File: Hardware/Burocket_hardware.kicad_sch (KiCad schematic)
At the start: 0 parts

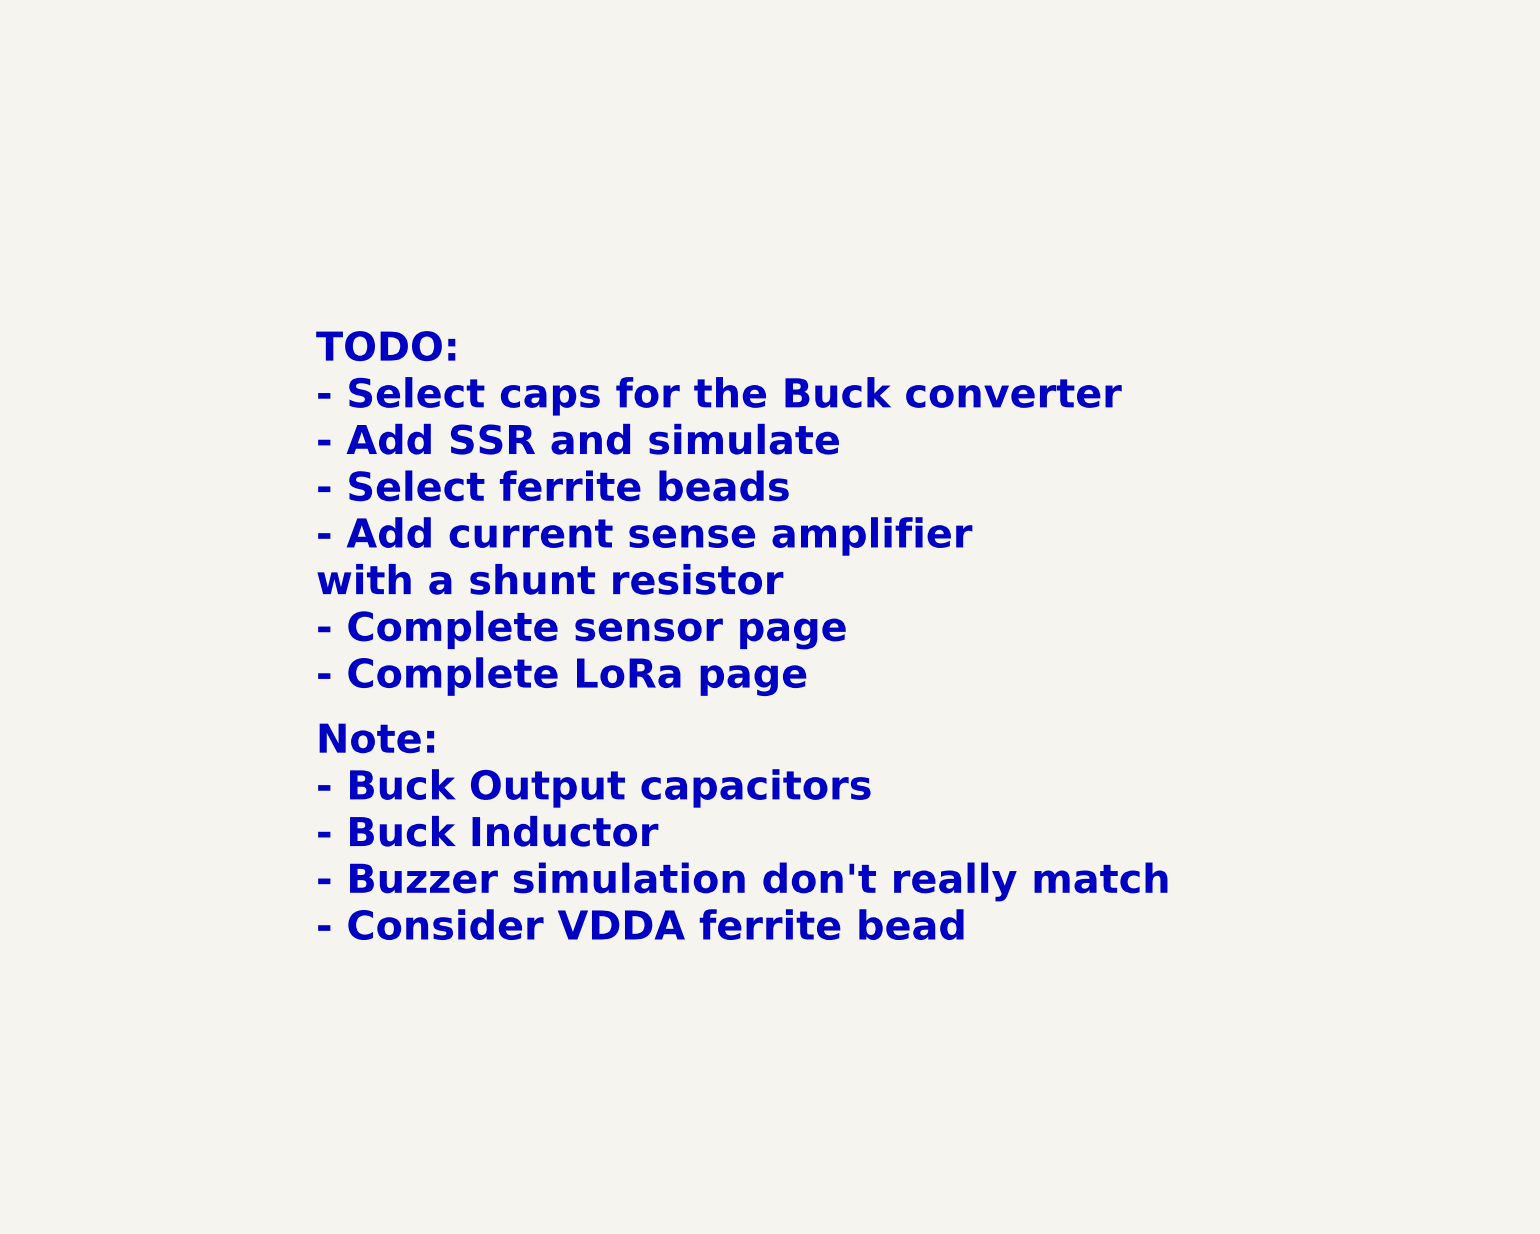
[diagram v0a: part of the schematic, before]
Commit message: Commit bulamadim :)
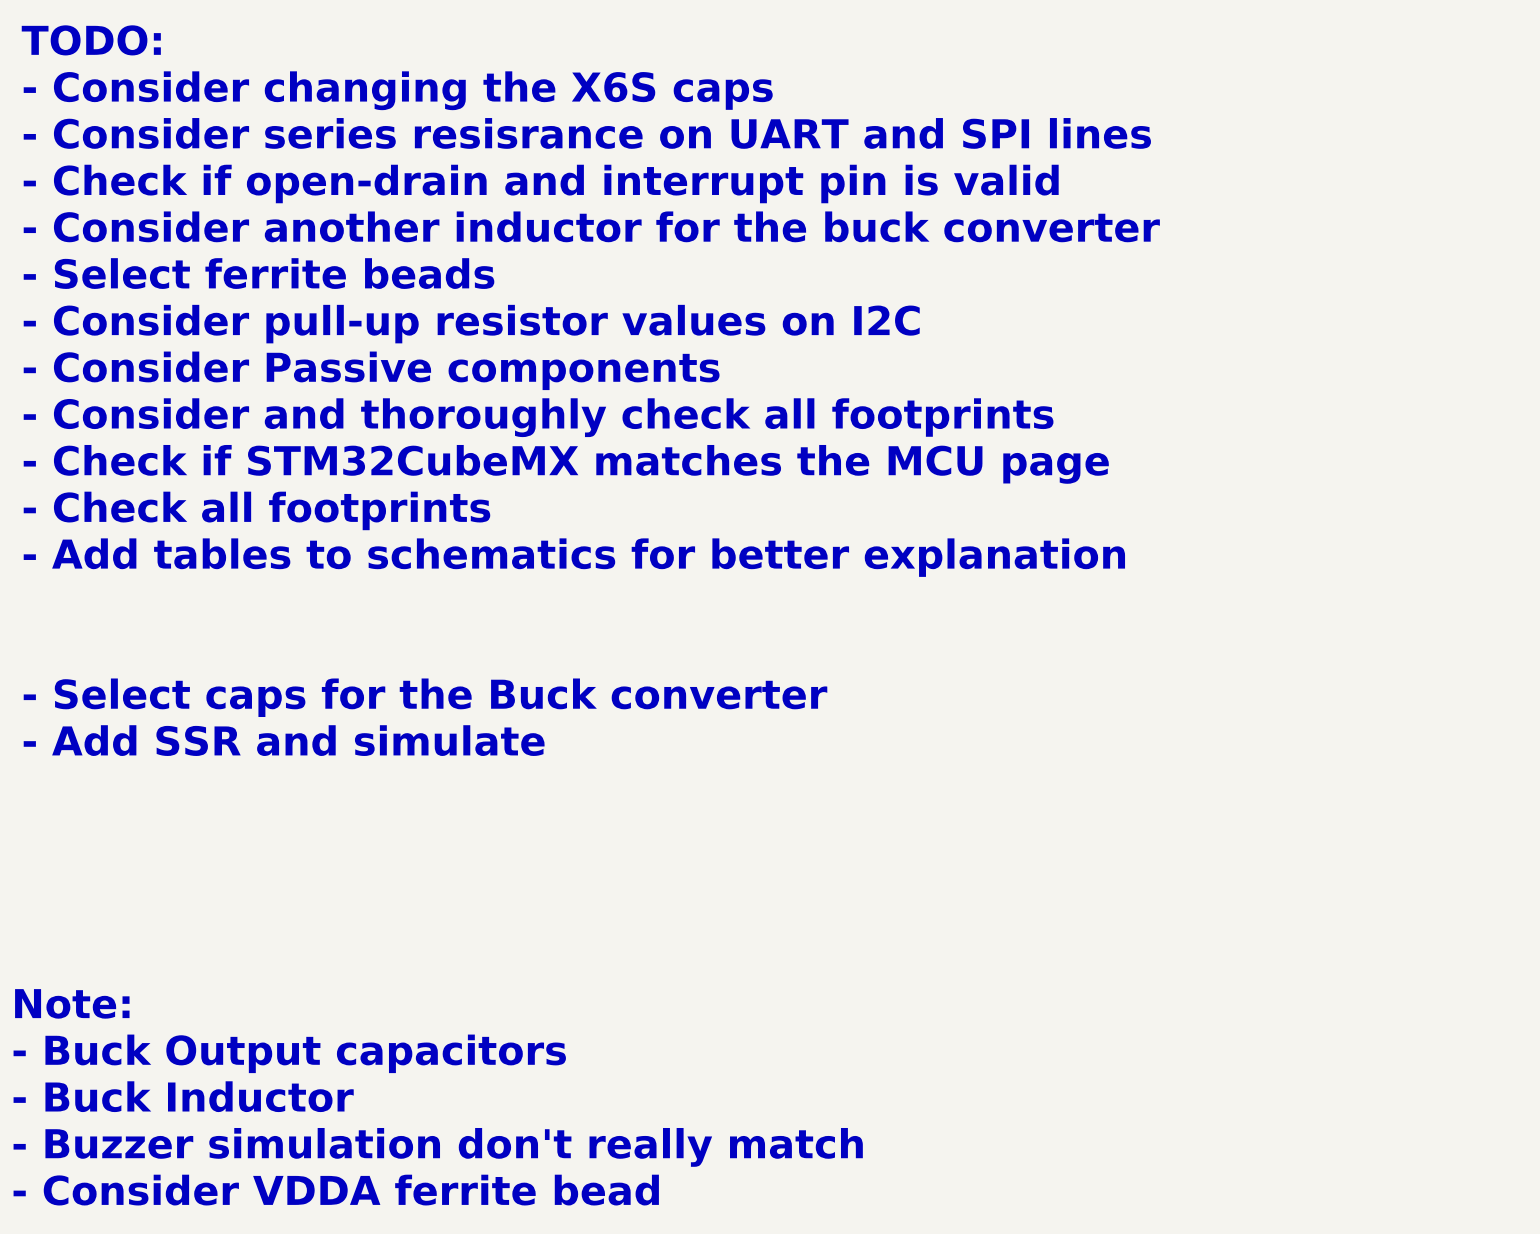
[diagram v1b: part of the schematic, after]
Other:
- note added: "TODO: - Consider changing the X6S caps - Consider series resisrance on UART and SPI lines - Check if open-drain and interrupt pin is valid - Consider another inductor for the buck converter - Select ferrite beads - Consider pull-up resistor values on I2C - Consider Passive components - Consider and thoroughly check all footprints - Check if STM32CubeMX matches the MCU page - Check all footprints 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"
- note removed: "TODO: - Select caps for the Buck converter - Add SSR and simulate - Select ferrite beads - Add current sense amplifier with a shunt resistor - Complete sensor page - Complete LoRa page"
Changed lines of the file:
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@@
 		(company "Burocket")
 	)
-	(text "TODO:\n- Select caps for the Buck converter\n- Add SSR and simulate\n- Select ferrite beads\n- Add current sense amplifier \nwith a shunt resistor\n- Complete sensor page\n- Complete LoRa page"
+	(text "TODO:\n- Consider changing the X6S caps\n- Consider series resisrance on UART and SPI lines\n- Check if open-drain and interrupt pin is valid\n- Consider another inductor for the buck converter\n- Select ferrite beads\n- Consider pull-up resistor values on I2C\n- Consider Passive components\n- Consider and thoroughly check all footprints\n- Check if STM32CubeMX matches the MCU page\n- Check all footprints\n- Add tables to schematics for better explanation\n\n\n- Select caps for the Buck converter\n- Add SSR and simulate"
 		(exclude_from_sim no)
-		(at -163.576 72.39 0)
+		(at -215.138 51.562 0)
 		(effects
 			(font
@@
 	(text "Note:\n- Buck Output capacitors\n- Buck Inductor\n- Buzzer simulation don't really match \n- Consider VDDA ferrite bead"
 		(exclude_from_sim no)
-		(at -163.576 128.778 0)
+		(at -216.916 175.26 0)
 		(effects
 			(font
